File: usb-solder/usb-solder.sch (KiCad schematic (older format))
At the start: 332 parts, among them J1 USB_B_Micro, J10 USB_B_Micro, J11 USB_B_Micro, J12 USB_B_Micro, J13 USB_B_Micro, J15 USB_B_Micro, J16 USB_B_Micro, J17 USB_B_Micro, J18 USB_B_Micro, J19 USB_B_Micro, J2 USB_B_Micro, J20 USB_B_Micro, J21 USB_B_Micro, J22 USB_B_Micro, J23 USB_A, J24 Conn_01x02_Male, J25 Barrel_Jack_Switch, J26 USB_B_Micro, J27 Conn_01x07_Male, J3 USB_B_Micro, J4 USB_B_Micro, J5 USB_B_Micro, J6 USB_B_Micro, J7 USB_B_Micro, J8 USB_B_Micro, J9 USB_B_Micro, SW1 SW_SPDT, U1 555, U2 74HC164, U3 4072, U4 74AHC1G04, U5 AP1117-33

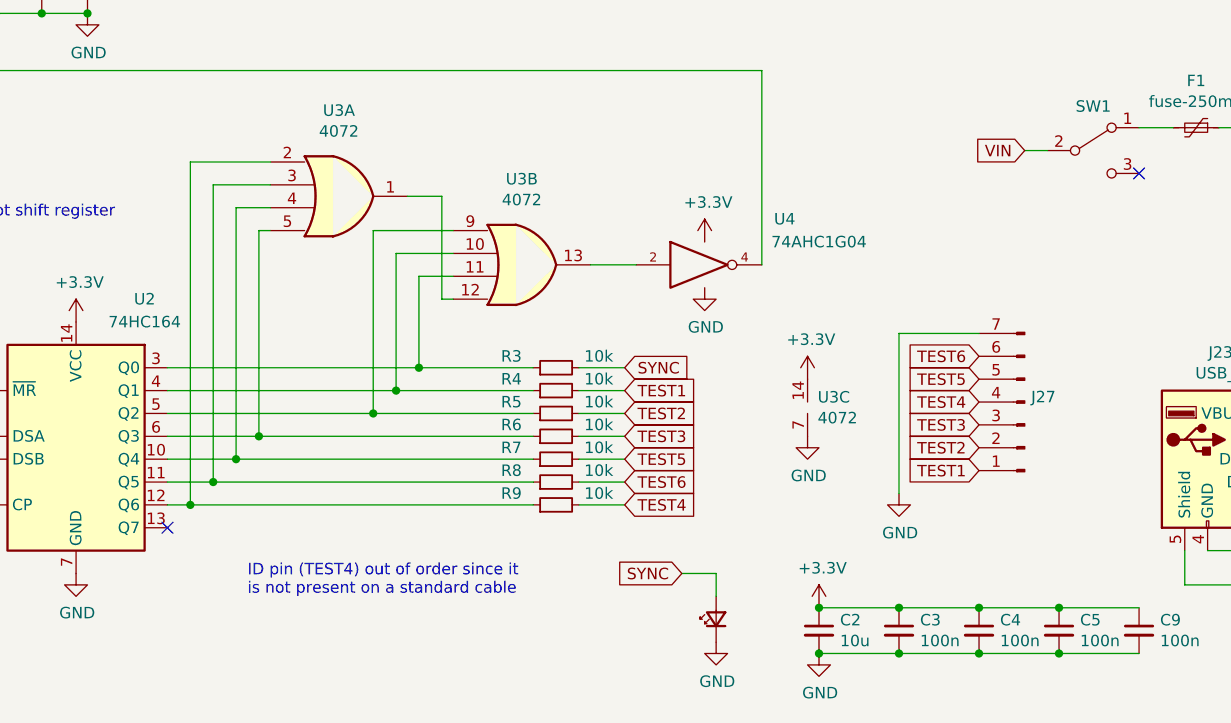
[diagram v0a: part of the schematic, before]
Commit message: v1
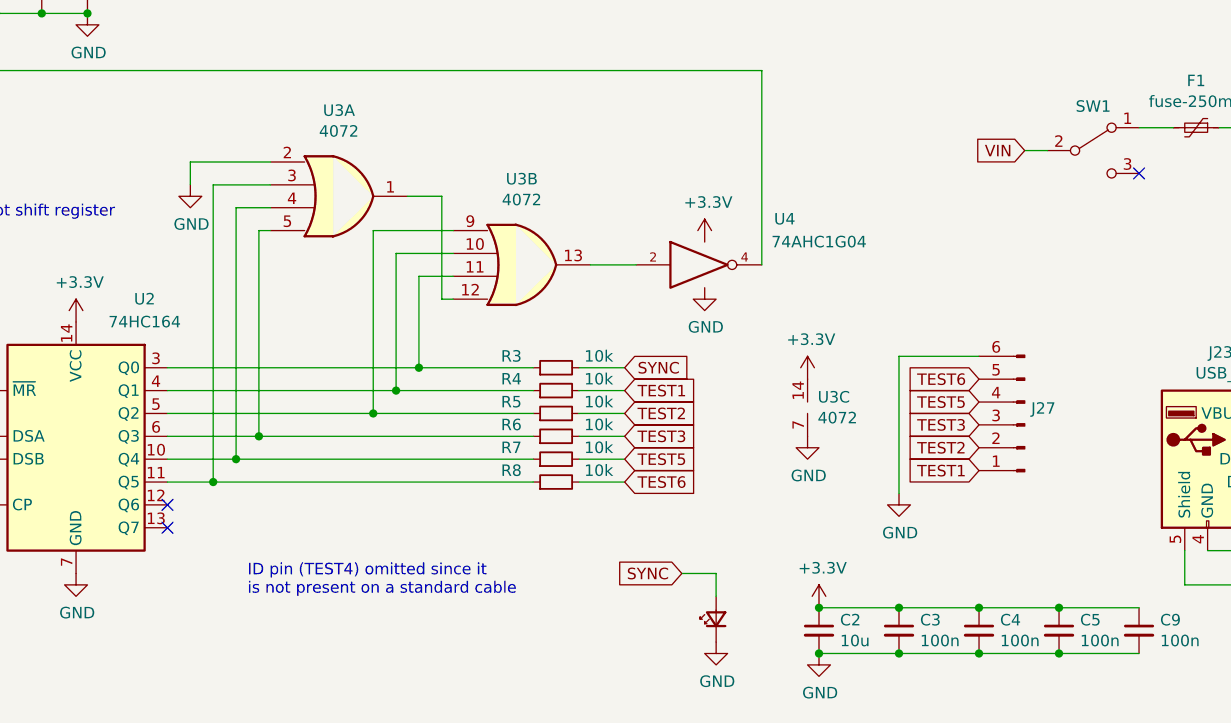
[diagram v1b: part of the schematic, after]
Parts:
- removed J27: Conn_01x07_Male, Connector_PinHeader_2.54mm:PinHeader_1x07_P2.54mm_Vertical, symbol pace:Conn_01x07_Male
- removed R9: 10k, Resistor_SMD:R_0402_1005Metric, symbol pace:10k
- added J27: Conn_01x06_Male, Connector_PinHeader_2.54mm:PinHeader_1x06_P2.54mm_Vertical, symbol pace:Conn_01x06_Male
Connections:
- net GND: now also U3.2, J27.6 (Pin_6)
- net TEST1: now also J27.1 (Pin_1)
- net TEST2: now also J27.2 (Pin_2)
- net TEST3: now also J27.3 (Pin_3)
- net TEST5: now also J27.4 (Pin_4)
- net TEST6: now also J27.5 (Pin_5)
- net at U2.12 (Q6): no longer U3.2
- no-connect marks 6 -> 7
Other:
- note added: "ID pin (TEST4) omitted since it\nis not present on a standard cable"
- note removed: "ID pin (TEST4) out of order since it\nis not present on a standard cable"
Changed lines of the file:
@@
 	0    -1   -1   0
 $EndComp
-Text GLabel 6300 7350 2    50   Input ~ 0
-TEST4
 Text GLabel 9700 6950 2    50   Input ~ 0
 TEST1
@@
 TEST3
 Text GLabel 7850 6900 0    50   Input ~ 0
-TEST4
+TEST5
 Text GLabel 7850 6800 0    50   Input ~ 0
-TEST5
-Text GLabel 7850 6700 0    50   Input ~ 0
 TEST6
-$Comp
-L pace:Conn_01x07_Male J27
-U 1 1 60AD63DE
-P 8050 6900
-F 0 "J27" H 8022 6878 50  0000 R CNN
-F 1 "Conn_01x07_Male" H 8022 6923 50  0001 R CNN
-F 2 "Connector_PinHeader_2.54mm:PinHeader_1x07_P2.54mm_Vertical" H 8050 6900 50  0001 C CNN
-F 3 "~" H 8050 6900 50  0001 C CNN
-	1    8050 6900
-	-1   0    0    1
-$EndComp
 $Comp
 L pace:GND #PWR?
@@
 $EndComp
 Wire Wire Line
-	7850 6600 7500 6600
-Wire Wire Line
-	7500 6600 7500 7300
+	7850 6700 7500 6700
+Wire Wire Line
+	7500 6700 7500 7300
 Text Notes 4650 7750 0    50   ~ 0
-ID pin (TEST4) out of order since it\nis not present on a standard cable
+ID pin (TEST4) omitted since it\nis not present on a standard cable
 Text Notes 850  6400 0    50   ~ 0
 200 millisec period clock
@@
 $EndComp
 NoConn ~ 8550 5900
-$Comp
-L pace:10k R9
-U 1 1 6028FF76
-P 6000 7350
-F 0 "R9" V 6050 7500 50  0000 L CNN
-F 1 "10k" V 6050 7100 50  0000 L CNN
-F 2 "Resistor_SMD:R_0402_1005Metric" H 6000 7350 50  0001 C CNN
-F 3 "https://datasheet.lcsc.com/szlcsc/Uniroyal-Elec-0402WGF1002TCE_C25744.pdf" H 6000 7350 50  0001 C CNN
-F 4 "C25744" H 6000 7350 50  0001 C CNN "LCSC"
-	1    6000 7350
-	0    -1   -1   0
-$EndComp
 Wire Wire Line
 	6700 7650 6700 7750
@@
 Wire Wire Line
 	6100 7250 6300 7250
-Wire Wire Line
-	6100 7350 6300 7350
 Wire Wire Line
 	6900 6300 6900 5450
@@
 	4300 7250 4500 7250
 Wire Wire Line
-	4300 7350 4400 7350
-Wire Wire Line
-	4400 5850 4400 7350
-Connection ~ 4400 7350
-Wire Wire Line
-	4400 7350 5900 7350
-Wire Wire Line
 	4500 5950 4500 7250
 Connection ~ 4500 7250
@@
 Connection ~ 8250 2250
 Connection ~ 8250 3200
+NoConn ~ 4300 7350
+$Comp
+L pace:GND #PWR?
+U 1 1 5FEECE60
+P 4400 5950
+F 0 "#PWR?" H 4400 5700 50  0001 C CNN
+F 1 "GND" H 4405 5777 50  0000 C CNN
+F 2 "" H 4400 5950 50  0001 C CNN
+F 3 "" H 4400 5950 50  0001 C CNN
+	1    4400 5950
+	1    0    0    -1
+$EndComp
+Wire Wire Line
+	4400 5850 4400 5950
+$Comp
+L pace:Conn_01x06_Male J27
+U 1 1 5FF4CAD5
+P 8050 7000
+F 0 "J27" H 8022 6928 50  0000 R CNN
+F 1 "Conn_01x06_Male" H 8022 6973 50  0001 R CNN
+F 2 "Connector_PinHeader_2.54mm:PinHeader_1x06_P2.54mm_Vertical" H 8050 7000 50  0001 C CNN
+F 3 "~" H 8050 7000 50  0001 C CNN
+	1    8050 7000
+	-1   0    0    1
+$EndComp
 $EndSCHEMATC
